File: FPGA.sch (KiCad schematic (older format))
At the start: 11 parts, among them U14 SiT8008B, U8 GW1N-9LQ100

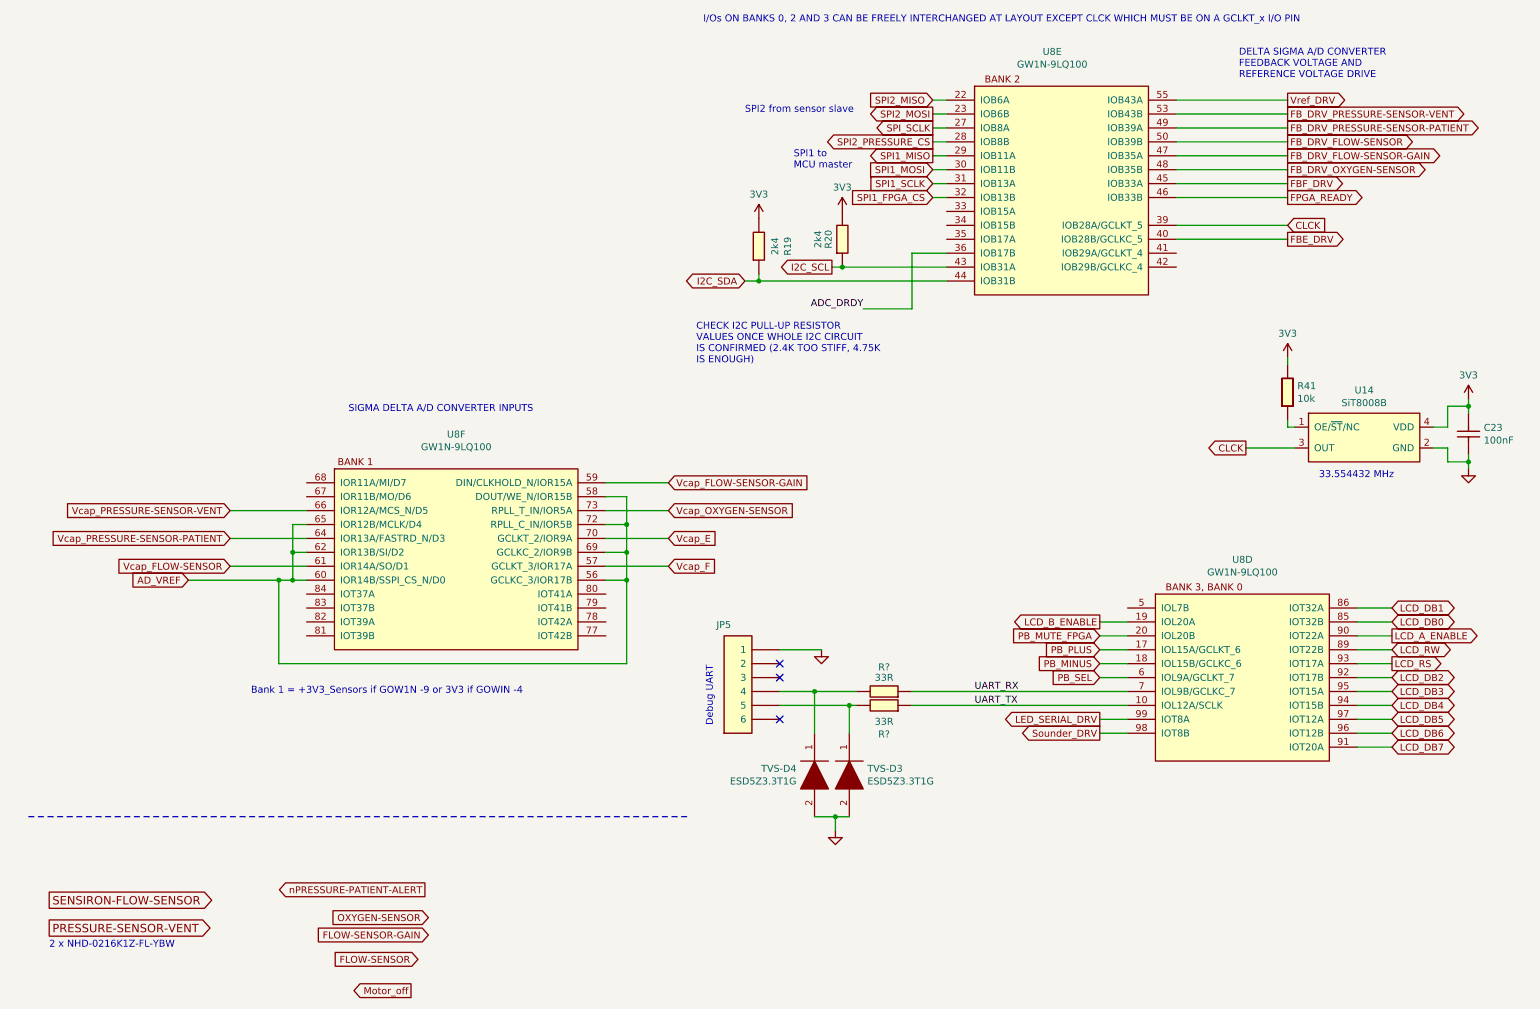
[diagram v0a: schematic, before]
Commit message: Update FPGA.sch
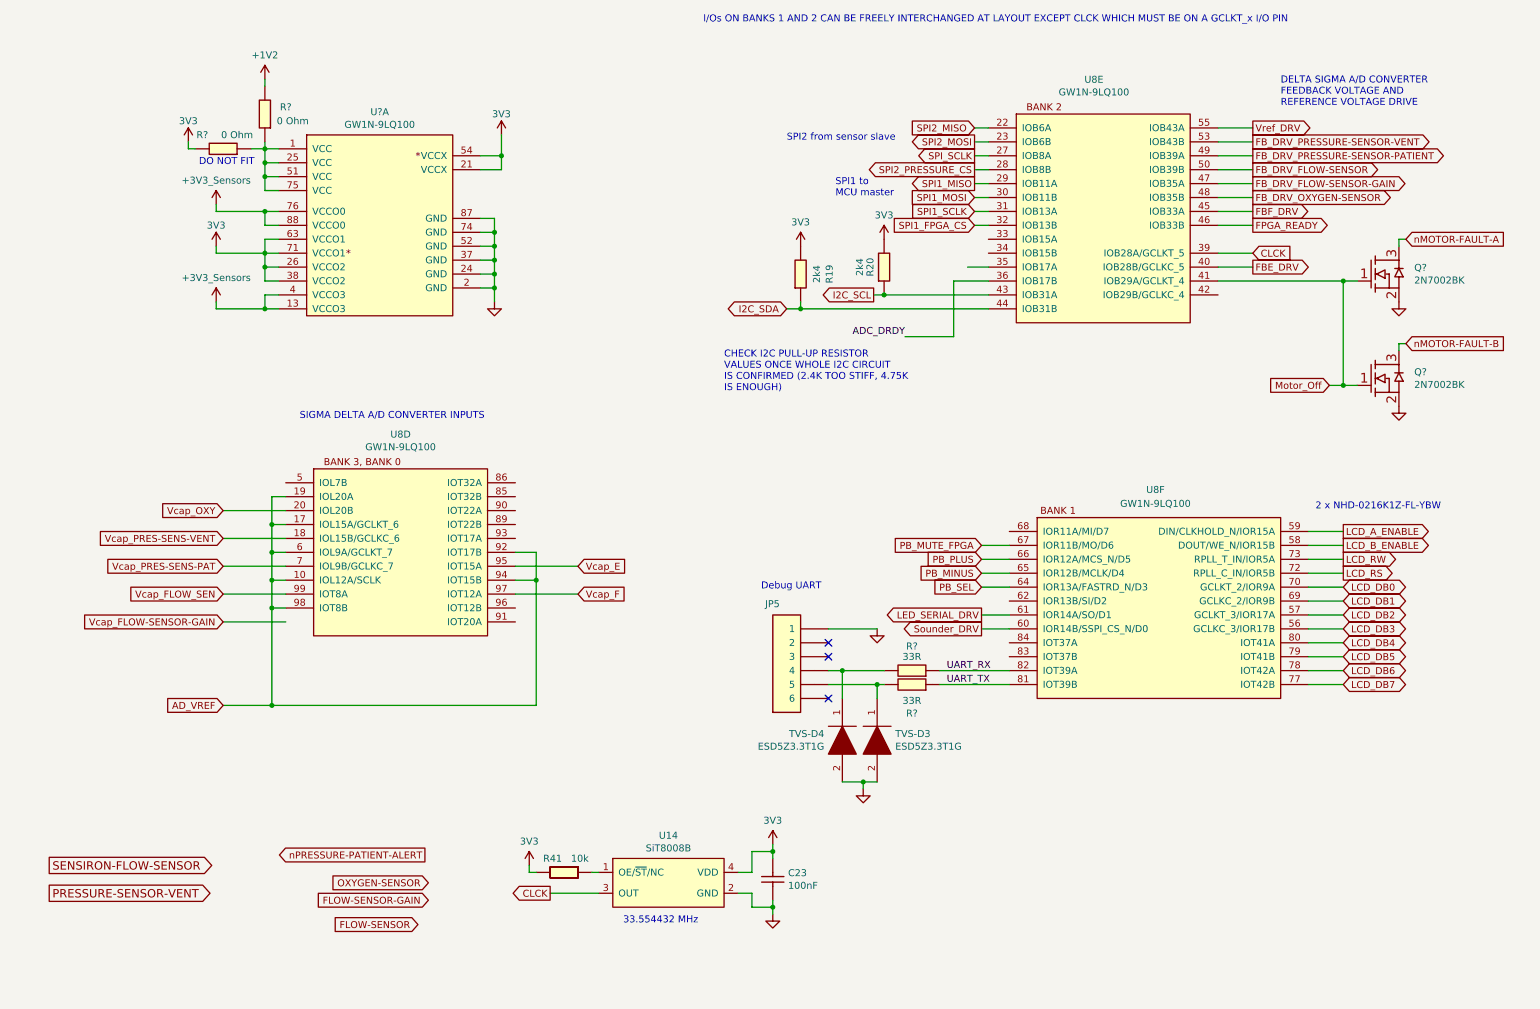
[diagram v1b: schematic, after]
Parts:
- added Q? (x2): 2N7002BK, symbol OpenVent:2N7002BK
- added R? (x2): 0R0_0603_Chip_Resistor,_1%,_0.1W, symbol OpenVent:0R0_0603_Chip_Resistor,_1%,_0.1W
- added U?: GW1N-9LQ100, symbol OpenVent:GW1N-9LQ100
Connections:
- net Vcap_FLOW-SENSOR is gone; now on net LED_SERIAL_DRV: U8.61 (IOR14A/SO/D1)
- net Vcap_OXYGEN-SENSOR is gone; now on net LCD_RW: U8.73 (RPLL_T_IN/IOR5A)
- net Vcap_PRESSURE-SENSOR-PATIENT is gone; now on net PB_SEL: U8.64 (IOR13A/FASTRD_N/D3)
- net Vcap_PRESSURE-SENSOR-VENT is gone; now on net PB_PLUS: U8.66 (IOR12A/MCS_N/D5)
- net +3V3: now also R?.2, U?.21 (VCCX), U?.26 (VCCO2), U?.38 (VCCO2), U?.54 (VCCX), U?.63 (VCCO1), U?.71 (VCCO1)
- net AD_VREF: now also U8.10 (IOL12A/SCLK), U8.17 (IOL15A/GCLKT_6), U8.19 (IOL20A), U8.6 (IOL9A/GCLKT_7), U8.92 (IOT17B), U8.94 (IOT15B), U8.98 (IOT8B); no longer U8.56 (GCLKC_3/IOR17B), U8.58 (DOUT/WE_N/IOR15B), U8.60 (IOR14B/SSPI_CS_N/D0), U8.62 (IOR13B/SI/D2), U8.65 (IOR12B/MCLK/D4), U8.69 (GCLKC_2/IOR9B), U8.72 (RPLL_C_IN/IOR5B)
- net GND: now also Q?.2 (S), Q?.2 (S), U?.2 (GND), U?.24 (GND), U?.37 (GND), U?.52 (GND), U?.74 (GND), U?.87 (GND)
- net LCD_A_ENABLE: now also U8.59 (DIN/CLKHOLD_N/IOR15A); no longer U8.90 (IOT22A)
- net LCD_B_ENABLE: now also U8.58 (DOUT/WE_N/IOR15B); no longer U8.19 (IOL20A)
- net LCD_DB0: now also U8.70 (GCLKT_2/IOR9A); no longer U8.85 (IOT32B)
- net LCD_DB1: now also U8.69 (GCLKC_2/IOR9B); no longer U8.86 (IOT32A)
- net LCD_DB2: now also U8.57 (GCLKT_3/IOR17A); no longer U8.92 (IOT17B)
- net LCD_DB3: now also U8.56 (GCLKC_3/IOR17B); no longer U8.95 (IOT15A)
- net LCD_DB4: now also U8.80 (IOT41A); no longer U8.94 (IOT15B)
- net LCD_DB5: now also U8.79 (IOT41B); no longer U8.97 (IOT12A)
- net LCD_DB6: now also U8.78 (IOT42A); no longer U8.96 (IOT12B)
- net LCD_DB7: now also U8.77 (IOT42B); no longer U8.91 (IOT20A)
- net LCD_RS: now also U8.72 (RPLL_C_IN/IOR5B); no longer U8.93 (IOT17A)
- net LCD_RW: no longer U8.89 (IOT22B)
- net LED_SERIAL_DRV: no longer U8.99 (IOT8A)
- net PB_MINUS: now also U8.65 (IOR12B/MCLK/D4); no longer U8.18 (IOL15B/GCLKC_6)
- net PB_MUTE_FPGA: now also U8.67 (IOR11B/MO/D6); no longer U8.20 (IOL20B)
- net PB_PLUS: no longer U8.17 (IOL15A/GCLKT_6)
- net PB_SEL: no longer U8.6 (IOL9A/GCLKT_7)
- net Sounder_DRV: now also U8.60 (IOR14B/SSPI_CS_N/D0); no longer U8.98 (IOT8B)
- net UART_RX: now also U8.82 (IOT39A); no longer U8.7 (IOL9B/GCLKC_7)
- net UART_TX: now also U8.81 (IOT39B); no longer U8.10 (IOL12A/SCLK)
- net Vcap_E: now also U8.95 (IOT15A); no longer U8.70 (GCLKT_2/IOR9A)
- net Vcap_F: now also U8.97 (IOT12A); no longer U8.57 (GCLKT_3/IOR17A)
- net Vcap_FLOW-SENSOR-GAIN: no longer U8.59 (DIN/CLKHOLD_N/IOR15A)
- net Motor_Off: now reaches U8.41 (IOB29A/GCLKT_4)
- net Motor_Off: now also Q?.1 (G1), Q?.1 (G1)
- new net: R?.1, R?.1, U?.1 (VCC), U?.25 (VCC), U?.51 (VCC), U?.75 (VCC)
- new net +3.3V: U?.13 (VCCO3), U?.4 (VCCO3), U?.76 (VCCO0), U?.88 (VCCO0)
- new net +5V: R?.2
- new net Vcap_FLOW_SEN: U8.99 (IOT8A)
- new net Vcap_OXY: U8.20 (IOL20B)
- new net Vcap_PRES-SENS-PAT: U8.7 (IOL9B/GCLKC_7)
- new net Vcap_PRES-SENS-VENT: U8.18 (IOL15B/GCLKC_6)
- new net nMOTOR-FAULT-A: Q?.3 (D)
- new net nMOTOR-FAULT-B: Q?.3 (D)
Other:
- note added: "DO NOT FIT"
- note added: "I/Os ON BANKS 1 AND 2 CAN BE FREELY INTERCHANGED AT LAYOUT EXCEPT CLCK WHICH MUST BE ON A GCLKT_x I/O PIN"
- note removed: "Bank 1 = +3V3_Sensors if GOW1N -9 or 3V3 if GOWIN -4"
- note removed: "I/Os ON BANKS 0, 2 AND 3 CAN BE FREELY INTERCHANGED AT LAYOUT EXCEPT CLCK WHICH MUST BE ON A GCLKT_x I/O PIN"
- moved on the sheet: C23, JP5, R19, R20, R41, R?, TVS-D3, TVS-D4, U14, U8D, U8E, U8F

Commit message: Update FPGA.sch
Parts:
- U8, U?: symbol OpenVent:GW1N-9LQ100 -> OpenVent-rescue:GW1N-9LQ100-OpenVent
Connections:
- net AD_VREF: now also U8.86 (IOT32A), U8.90 (IOT22A), U8.97 (IOT12A), U8.99 (IOT8A); no longer U8.10 (IOL12A/SCLK), U8.92 (IOT17B), U8.94 (IOT15B), U8.98 (IOT8B)
- net Vcap_E: now also U8.89 (IOT22B); no longer U8.95 (IOT15A)
- net Vcap_F: now also U8.85 (IOT32B); no longer U8.97 (IOT12A)
- net Vcap_FLOW-SENSOR-GAIN: now also U8.96 (IOT12B)
- net Vcap_FLOW_SEN: now also U8.98 (IOT8B); no longer U8.99 (IOT8A)
- net Vcap_OXY: now also U8.7 (IOL9B/GCLKC_7); no longer U8.20 (IOL20B)
- net Vcap_PRES-SENS-PAT: now also U8.20 (IOL20B); no longer U8.7 (IOL9B/GCLKC_7)
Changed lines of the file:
@@
 	7400 2100 7300 2100
 $Comp
-L OpenVent:GW1N-9LQ100 U8
+L OpenVent-rescue:GW1N-9LQ100-OpenVent U8
 U 6 1 6053AF87
 P 8600 4200
@@
 Connection ~ 3900 1600
 $Comp
-L OpenVent:GW1N-9LQ100 U?
+L OpenVent-rescue:GW1N-9LQ100-OpenVent U?
 U 1 1 605DEC3D
 P 3000 1450
 AR Path="/5FBE8499/605DEC3D" Ref="U?"  Part="1"
 AR Path="/5F8F894A/605DEC3D" Ref="U?"  Part="1"
+AR Path="/605DEC3D" Ref="U?"  Part="1"
 F 0 "U?" H 3025 1615 50  0000 C CNN
 F 1 "GW1N-9LQ100" H 3025 1524 50  0000 C CNN
@@
 	6650 2600 7400 2600
 $Comp
-L OpenVent:GW1N-9LQ100 U8
+L OpenVent-rescue:GW1N-9LQ100-OpenVent U8
 U 4 1 60544613
 P 3200 3850
@@
 	7400 2400 7250 2400
 $Comp
-L OpenVent:GW1N-9LQ100 U8
+L OpenVent-rescue:GW1N-9LQ100-OpenVent U8
 U 5 1 6054191D
 P 8200 1300
